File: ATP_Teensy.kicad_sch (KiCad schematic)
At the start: 7 parts

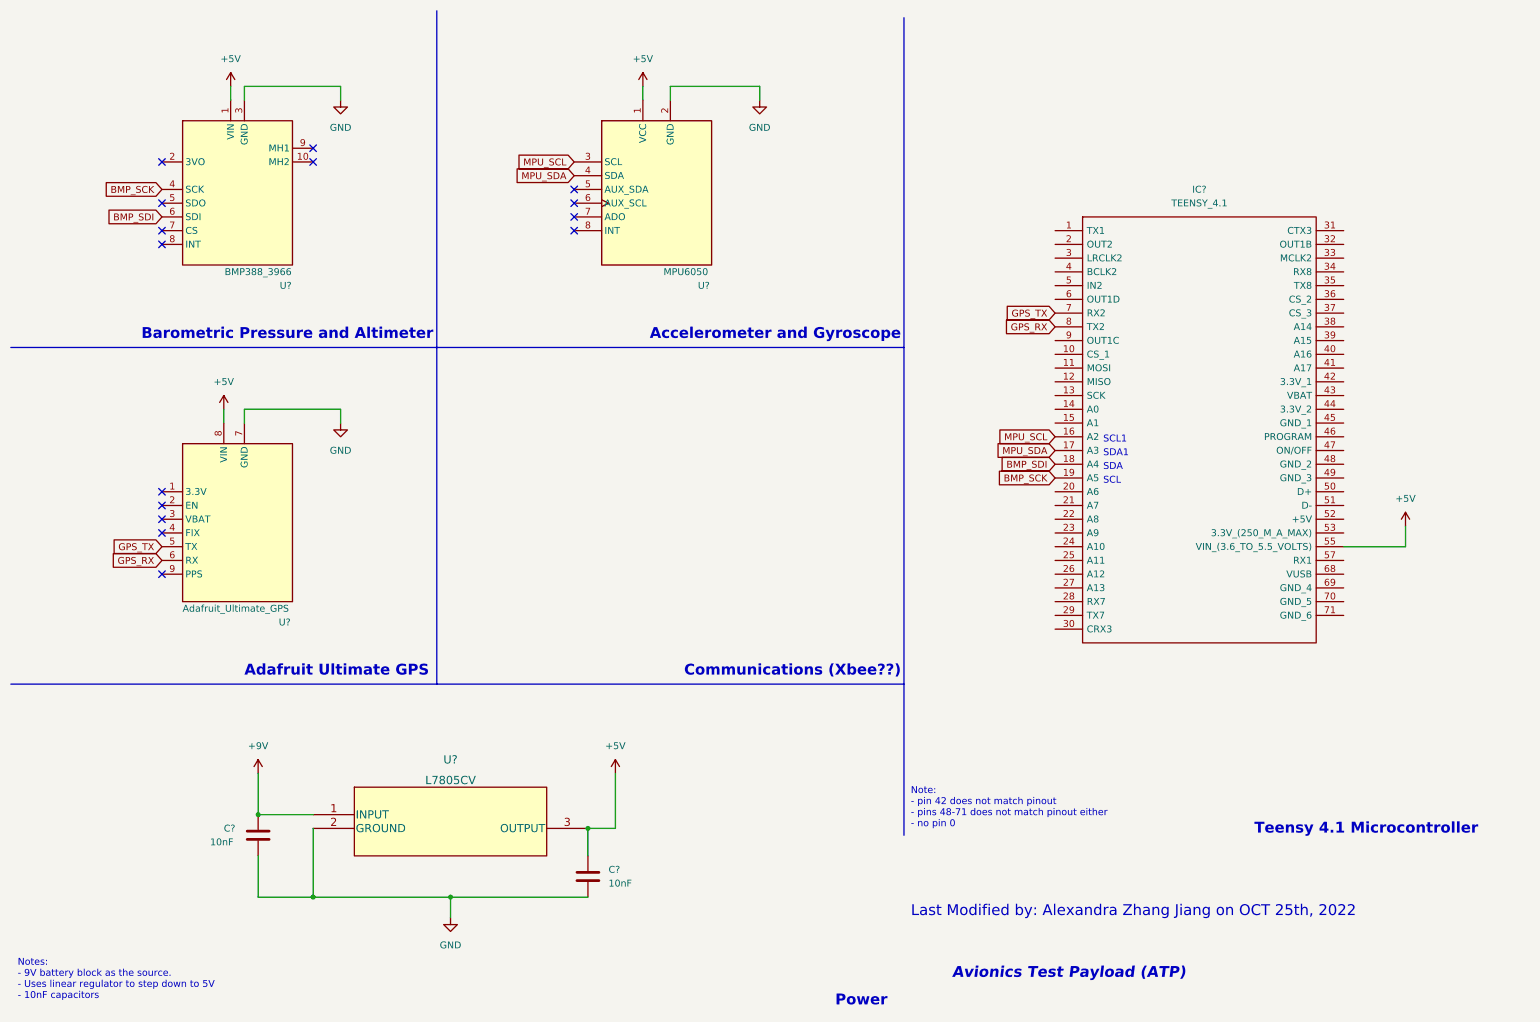
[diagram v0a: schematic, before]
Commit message: add footprints
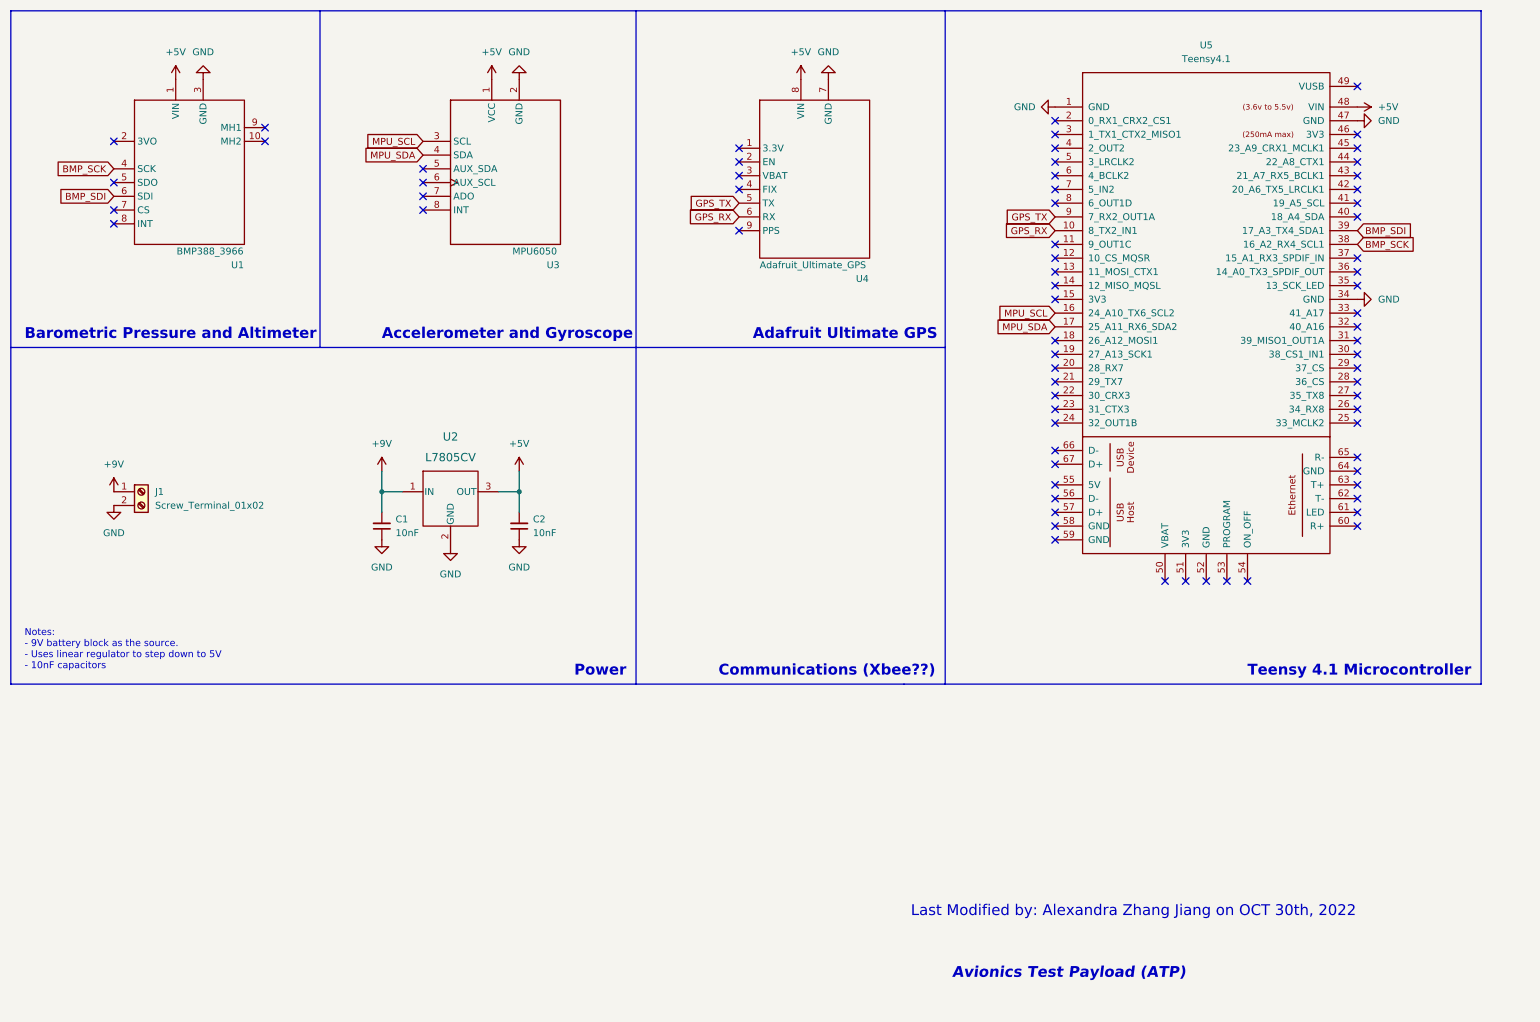
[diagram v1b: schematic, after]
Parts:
- removed C? (x2): 10nF, symbol Device:C
- removed IC?: TEENSY_4.1, TEENSY41, symbol ATP_Teensy-lib:TEENSY_4.1
- removed U?: Adafruit_Ultimate_GPS, symbol ATP_Teensy-lib:Adafruit_Ultimate_GPS
- removed U?: BMP388_3966, symbol ATP_Teensy-lib:BMP388_3966
- removed U?: L7805CV, TO-220_STM, symbol ATP_Teensy-lib:L7805CV
- removed U?: MPU6050, symbol ATP_Teensy-lib:MPU6050
- added C1, C2: 10nF, Capacitor_SMD:C_0805_2012Metric_Pad1.18x1.45mm_HandSolder, symbol Device:C_Small
- added J1: Screw_Terminal_01x02, TerminalBlock:TerminalBlock_bornier-2_P5.08mm, symbol Connector:Screw_Terminal_01x02
- added U1: BMP388_3966, Connector_PinSocket_2.54mm:PinSocket_1x08_P2.54mm_Vertical, symbol ATP_Teensy-lib:BMP388_3966
- added U2: L7805CV, ATP_Teensy_footprints:L7805CV, symbol ATP_Teensy-lib:L7805CV
- added U3: MPU6050, ATP_Teensy_footprints:IMU_board, symbol ATP_Teensy-lib:MPU6050
- added U4: Adafruit_Ultimate_GPS, ATP_Teensy_footprints:GPS_board, symbol ATP_Teensy-lib:Adafruit_Ultimate_GPS
- added U5: Teensy4.1, teensy:Teensy41, symbol teensy:Teensy4.1
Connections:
- net +5V: now also C2.2, U1.1 (VIN), U2.3 (OUT), U3.1 (VCC), U4.8 (VIN), U5.48 (VIN)
- net +9V: now also C1.2, J1.1 (Pin_1), U2.1 (IN)
- net BMP_SCK: now also U1.4 (SCK), U5.38 (16_A2_RX4_SCL1)
- net BMP_SDI: now also U1.6 (SDI), U5.39 (17_A3_TX4_SDA1)
- net GND: now also C1.1, C2.1, J1.2 (Pin_2), U1.3 (GND), U2.2 (GND), U3.2 (GND), U4.7 (GND), U5.1 (GND), U5.34 (GND), U5.47 (GND)
- net GPS_RX: now also U4.6 (RX), U5.10 (8_TX2_IN1)
- net GPS_TX: now also U4.5 (TX), U5.9 (7_RX2_OUT1A)
- net MPU_SCL: now also U3.3 (SCL), U5.16 (24_A10_TX6_SCL2)
- net MPU_SDA: now also U3.4 (SDA), U5.17 (25_A11_RX6_SDA2)
- no-connect marks 15 -> 72
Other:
- note added: "Last Modified by: Alexandra Zhang Jiang on OCT 30th, 2022"
- note removed: "Last Modified by: Alexandra Zhang Jiang on OCT 25th, 2022"
- note removed: "Note: - pin 42 does not match pinout - pins 48-71 does not match pinout either - no pin 0"
- note removed: "SCL"
- note removed: "SCL1"
- note removed: "SDA"
- note removed: "SDA1"
